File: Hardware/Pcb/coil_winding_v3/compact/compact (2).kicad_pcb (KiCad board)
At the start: 2 copper layers, 99.6 x 91.1 mm, 16 parts, among them J2 Screw_Terminal_01x02, J4 Conn_01x13_Socket, J6 Conn_01x05_Socket, M1 Motor_DC, Q3 IRFZ40, U1 LM7805_TO220

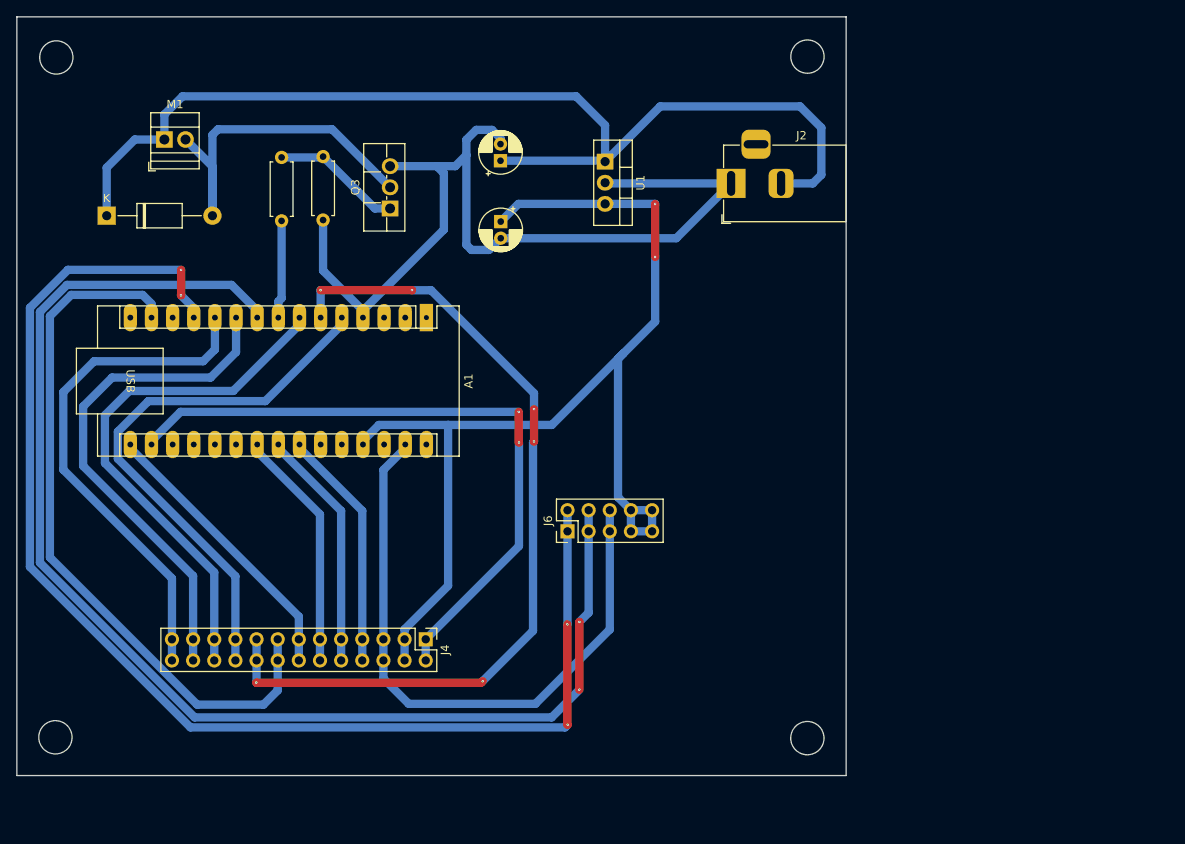
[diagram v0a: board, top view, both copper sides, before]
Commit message: final_code
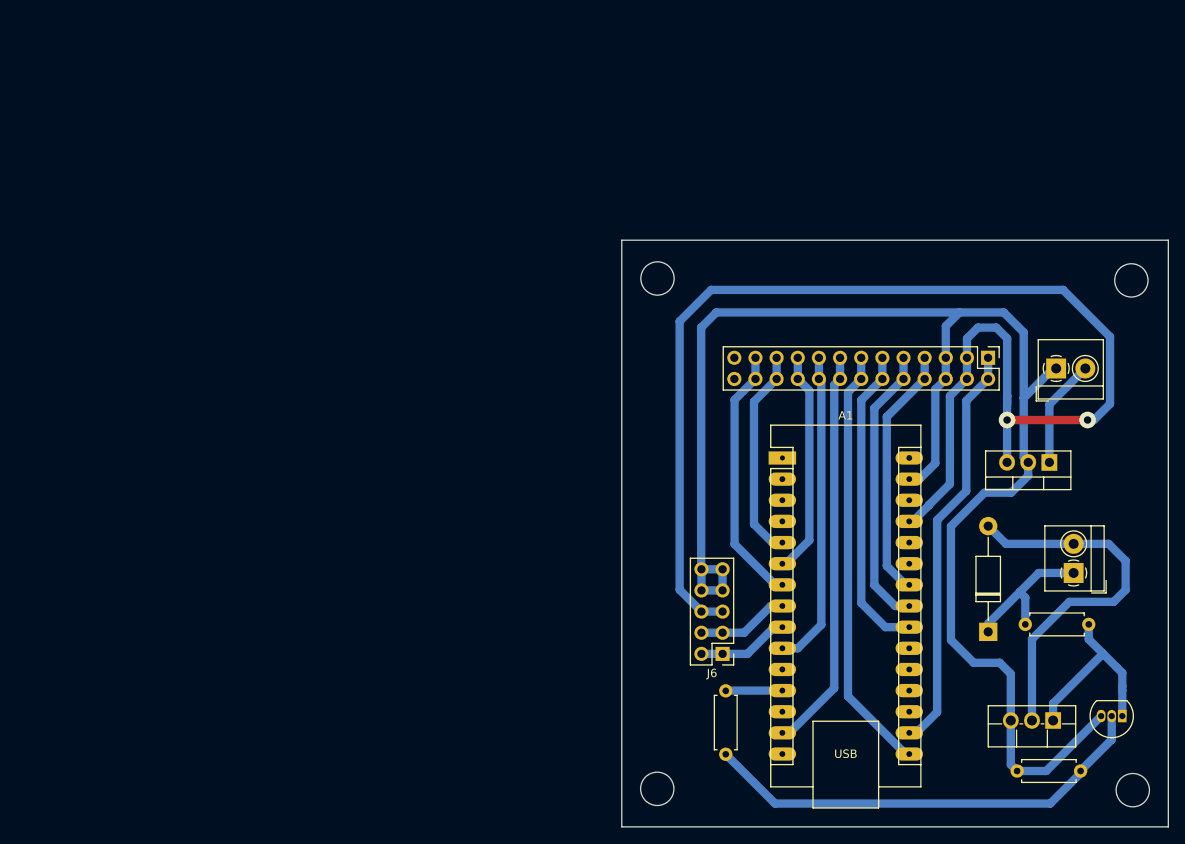
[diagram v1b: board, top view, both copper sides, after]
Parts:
- removed C1, C2: C, Capacitor_THT:CP_Radial_D5.0mm_P2.00mm
- added Q1: BC547, Package_TO_SOT_THT:TO-92_Inline, F.Cu at (179.0, 125.4)
- added R4: R, Resistor_THT:R_Axial_DIN0207_L6.3mm_D2.5mm_P7.62mm_Horizontal, F.Cu at (167.3, 114.4)
- J2: footprint Connector_BarrelJack:BarrelJack_Horizontal -> TerminalBlock_4Ucon:TerminalBlock_4Ucon_1x02_P3.50mm_Horizontal
- M1: footprint TerminalBlock:TerminalBlock_Xinya_XY308-2.54-2P_1x02_P2.54mm_Horizontal -> TerminalBlock_4Ucon:TerminalBlock_4Ucon_1x02_P3.50mm_Horizontal
- Q3: value IRFZ40 -> IRF540
- moved H4 131.9 mm to (180.1, 73.0)
- moved M1 121.0 mm to (173.1, 108.2), turned to 90 degrees
- moved D1 117.1 mm to (162.9, 115.3), turned to 90 degrees
- moved R2 106.4 mm to (166.4, 132.0), turned to 0 degrees
- moved Q3 100.6 mm to (170.7, 125.9), turned to 180 degrees
- moved H1 96.4 mm to (180.2, 134.3)
- moved R1 77.7 mm to (131.4, 122.3), turned to -90 degrees
- moved J4 75.5 mm to (162.9, 82.3)
- moved H2 72.6 mm to (123.1, 134.1)
- moved U1 64.4 mm to (170.2, 94.9), turned to 180 degrees
- moved H3 58.1 mm to (123.2, 72.8)
- moved A1 46.0 mm to (138.2, 94.4), turned to 0 degrees
- moved J2 44.9 mm to (171.1, 83.6), turned to 0 degrees
- moved J6 23.7 mm to (131.0, 117.9), turned to 180 degrees
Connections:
- D1 pad 1: VCC -> Net-(D1-K)
- J4 pad 10: D2 -> D3
- J4 pad 11: D4 -> D2
- J4 pad 12: D7 -> D4
- J4 pad 13: D8 -> unconnected-(J4-Pin_13-Pad13)
- J4 pad 9: D3 -> D7
- J6 pad 1: D9 -> D6
- J6 pad 2: D6 -> D5
- J6 pad 3: GND -> +5V
- J6 pad 4: +5V -> GND
- J6 pad 5: +5V -> GND
- M1 pad 1: VCC -> Net-(D1-K)
- Q3 pad 1: Net-(Q3-G) -> Net-(Q1-C)
- R1 pad 1: D5 -> D9
- R1 pad 2: Net-(Q3-G) -> Net-(Q1-B)
- R2 pad 2: Net-(Q3-G) -> Net-(Q1-B)
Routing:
- net D9: track 156.1 -> 6.81 mm, vias 4 -> 0
- net D6: track 155.6 -> 11.0 mm, vias 2 -> 0
- net VCC: track 130.1 -> 13.1 mm
- net D3: track 103.7 -> 26.9 mm, vias 6 -> 0
- net D8: track 61.8 -> 0.00 mm
- net Net-(Q1-B): track 0.00 -> 55.0 mm
- net D2: track 66.4 -> 25.4 mm
- net D11: track 85.9 -> 48.4 mm
- net D4: track 63.6 -> 31.2 mm
- net 3V3: track 80.5 -> 49.5 mm, vias 2 -> 0
- net +5V: track 135.4 -> 162.3 mm
- net Net-(Q1-C): track 0.00 -> 23.2 mm
- net D7: track 61.2 -> 38.0 mm
- net Net-(D1-K): track 0.00 -> 17.9 mm
- net D13: track 34.3 -> 51.5 mm
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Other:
- board size 99.6 x 91.1 mm -> 65.7 x 70.5 mm
